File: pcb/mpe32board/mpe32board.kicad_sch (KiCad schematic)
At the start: 42 parts, among them J1 Conn_ST_STDC14, J2 USB_C_Receptacle_USB2.0_16P, J46 Conn_02x10_Counter_Clockwise, SW1 SW_Push, SW2 SW_Push, U10 W9812G6KH-75, U2 USBLC6-2P6, U3 AMS1117-3.3, U9 STM32H743IITx

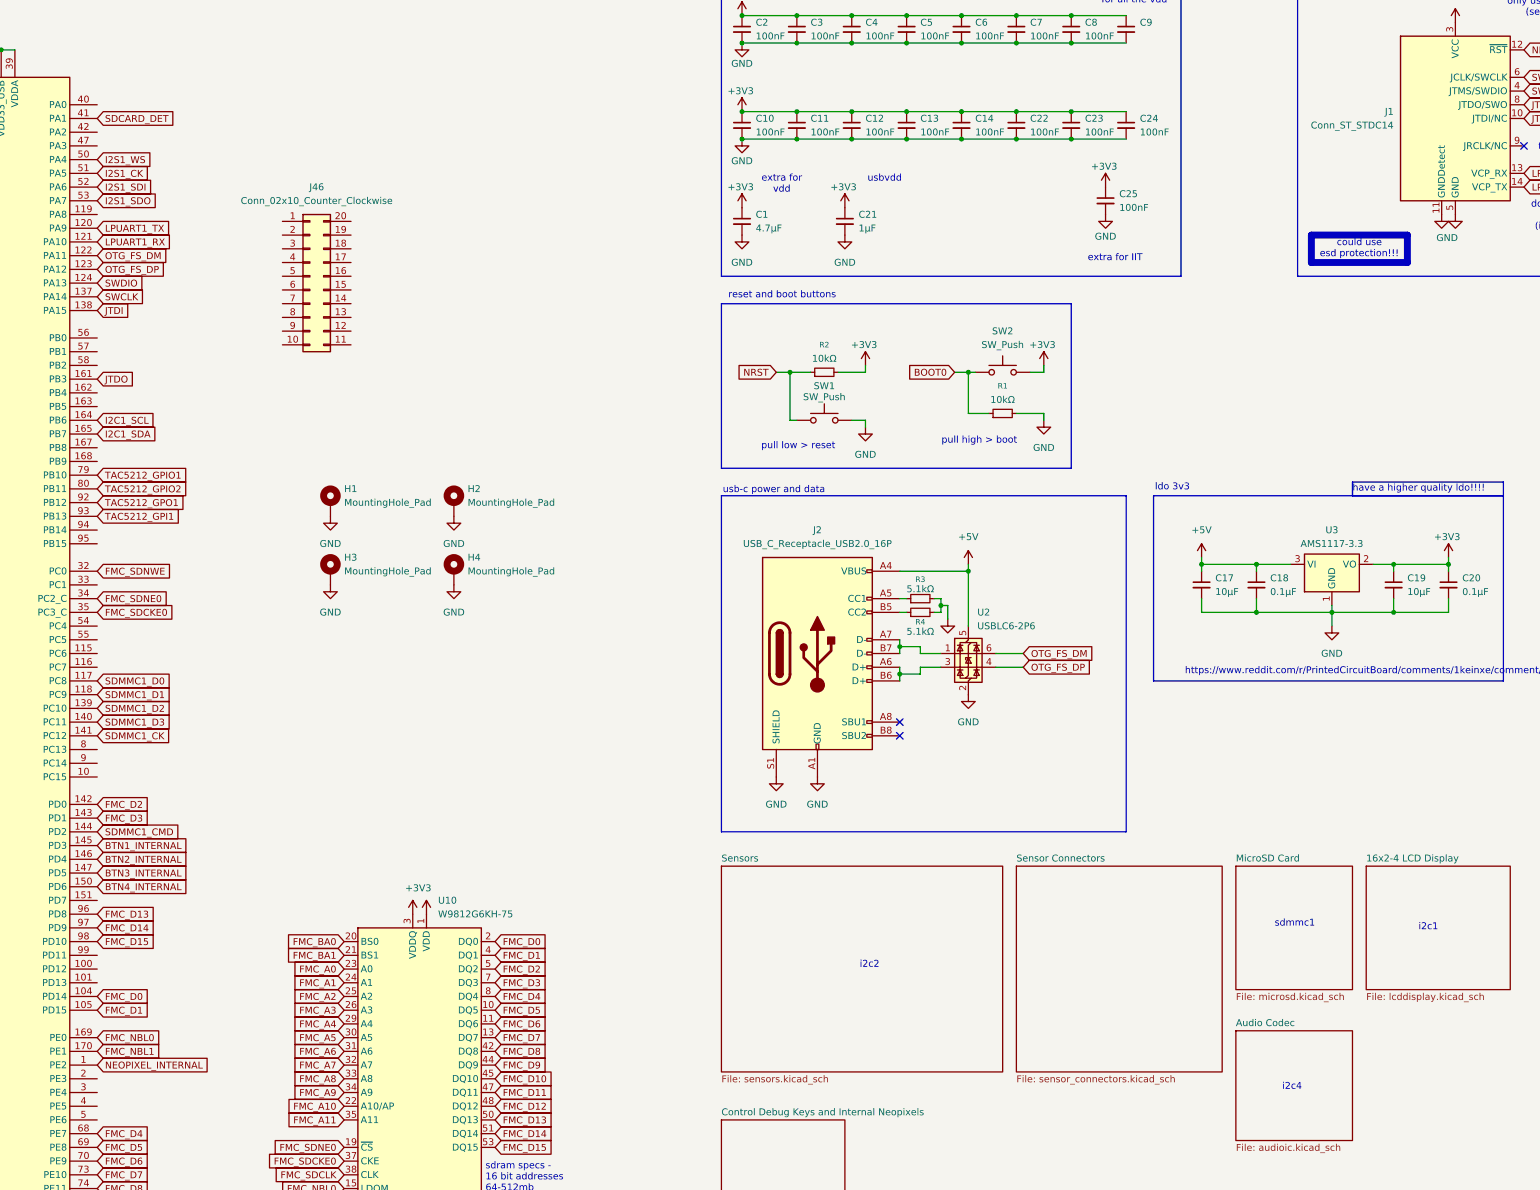
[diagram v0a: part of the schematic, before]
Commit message: routed ram
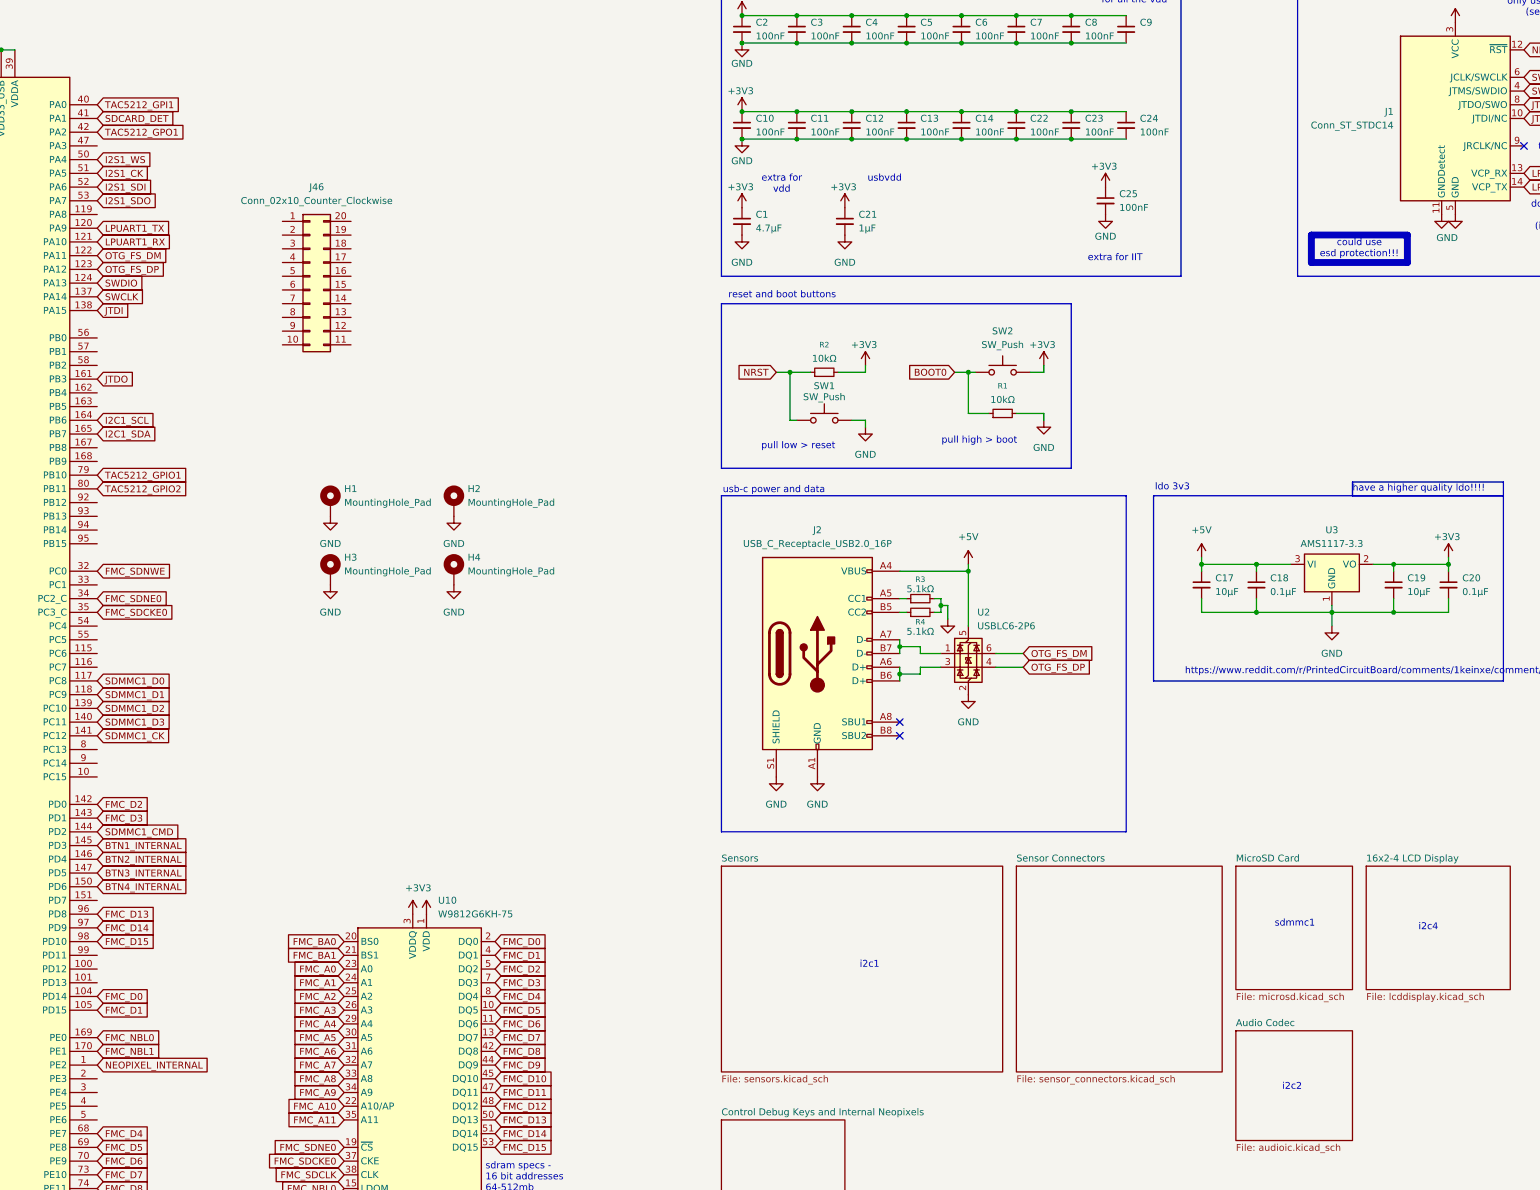
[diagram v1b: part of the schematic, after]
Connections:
- net TAC5212_GPI1: now also U9.40 (PA0); no longer U9.93 (PB13)
- net TAC5212_GPO1: now also U9.42 (PA2); no longer U9.92 (PB12)
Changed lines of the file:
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@@
 		)
 	)
-	(text "i2c4"
+	(text "i2c2\n"
 		(exclude_from_sim no)
 		(at 332.994 223.774 0)
@@
 		)
 	)
-	(text "i2c1"
+	(text "i2c4"
 		(exclude_from_sim no)
 		(at 358.2199 194.2105 0)
@@
 		)
 	)
-	(text "i2c2"
+	(text "i2c1"
 		(exclude_from_sim no)
 		(at 254.762 201.168 0)
@@
 		)
 	)
-	(global_label "FMC_D6"
+	(global_label "TAC5212_GPI1"
 		(shape input)
-		(at 111.76 237.49 0)
+		(at 111.76 41.91 0)
 		(fields_autoplaced yes)
 		(effects
@@
 		)
 		(property "Intersheetrefs" "${INTERSHEET_REFS}"
-			(at 122.0023 237.49 0)
+			(at 128.2313 41.91 0)
 			(hide yes)
 			(show_name no)
@@
 		)
 	)
-	(global_label "FMC_SDNCAS"
+	(global_label "FMC_D6"
 		(shape input)
-		(at 40.64 176.53 180)
+		(at 111.76 237.49 0)
 		(fields_autoplaced yes)
 		(effects
@@
 				(size 1.27 1.27)
 			)
-			(justify right)
+			(justify left)
 		)
 		(property "Intersheetrefs" "${INTERSHEET_REFS}"
-			(at 25.4991 176.53 0)
+			(at 122.0023 237.49 0)
 			(hide yes)
 			(show_name no)
@@
 					(size 1.27 1.27)
 				)
-				(justify right)
+				(justify left)
 			)
 		)
 	)
-	(global_label "NRST"
+	(global_label "FMC_SDNCAS"
 		(shape input)
-		(at 40.64 41.91 180)
+		(at 40.64 176.53 180)
 		(fields_autoplaced yes)
 		(effects
@@
 		)
 		(property "Intersheetrefs" "${INTERSHEET_REFS}"
-			(at 32.8772 41.91 0)
+			(at 25.4991 176.53 0)
 			(hide yes)
 			(show_name no)
@@
 		)
 	)
-	(global_label "TAC5212_GPI1"
+	(global_label "NRST"
 		(shape input)
-		(at 111.76 118.11 0)
+		(at 40.64 41.91 180)
 		(fields_autoplaced yes)
 		(effects
@@
 				(size 1.27 1.27)
 			)
-			(justify left)
+			(justify right)
 		)
 		(property "Intersheetrefs" "${INTERSHEET_REFS}"
-			(at 128.2313 118.11 0)
+			(at 32.8772 41.91 0)
 			(hide yes)
 			(show_name no)
@@
 					(size 1.27 1.27)
 				)
-				(justify left)
+				(justify right)
 			)
 		)
@@
 		)
 	)
-	(global_label "BTN3_INTERNAL"
+	(global_label "TAC5212_GPO1"
 		(shape input)
-		(at 111.76 184.15 0)
+		(at 111.76 46.99 0)
 		(fields_autoplaced yes)
 		(effects
@@
 		)
 		(property "Intersheetrefs" "${INTERSHEET_REFS}"
-			(at 129.2595 184.15 0)
+			(at 128.957 46.99 0)
 			(hide yes)
 			(show_name no)
@@
 		)
 	)
-	(global_label "BTN1_INTERNAL"
+	(global_label "BTN3_INTERNAL"
 		(shape input)
-		(at 111.76 179.07 0)
+		(at 111.76 184.15 0)
 		(fields_autoplaced yes)
 		(effects
@@
 		)
 		(property "Intersheetrefs" "${INTERSHEET_REFS}"
-			(at 129.2595 179.07 0)
+			(at 129.2595 184.15 0)
 			(hide yes)
 			(show_name no)
@@
 		)
 	)
-	(global_label "FMC_SDNWE"
+	(global_label "BTN1_INTERNAL"
 		(shape input)
-		(at 111.76 128.27 0)
+		(at 111.76 179.07 0)
 		(fields_autoplaced yes)
 		(effects
@@
 		)
 		(property "Intersheetrefs" "${INTERSHEET_REFS}"
-			(at 125.9332 128.27 0)
+			(at 129.2595 179.07 0)
 			(hide yes)
 			(show_name no)
@@
 		)
 	)
-	(global_label "FMC_D9"
+	(global_label "FMC_SDNWE"
 		(shape input)
-		(at 111.76 245.11 0)
+		(at 111.76 128.27 0)
 		(fields_autoplaced yes)
 		(effects
@@
 		)
 		(property "Intersheetrefs" "${INTERSHEET_REFS}"
-			(at 122.0023 245.11 0)
+			(at 125.9332 128.27 0)
 			(hide yes)
 			(show_name no)
@@
 		)
 	)
-	(global_label "TAC5212_GPO1"
+	(global_label "FMC_D9"
 		(shape input)
-		(at 111.76 115.57 0)
+		(at 111.76 245.11 0)
 		(fields_autoplaced yes)
 		(effects
@@
 		)
 		(property "Intersheetrefs" "${INTERSHEET_REFS}"
-			(at 128.957 115.57 0)
+			(at 122.0023 245.11 0)
 			(hide yes)
 			(show_name no)
